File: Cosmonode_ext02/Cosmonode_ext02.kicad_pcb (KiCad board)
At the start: 2 copper layers, 24.1 x 33 mm, 19 parts, among them J1 CONN_01X04, J2 CONN_01X04, J3 CONN_01X08, J4 CONN_01X08, J5 GS3, J6 GS3, Q1 BSS138, Q2 BSS138, SW1 SW_Push, SW2 SW_Push, U1 XC6206P502MR

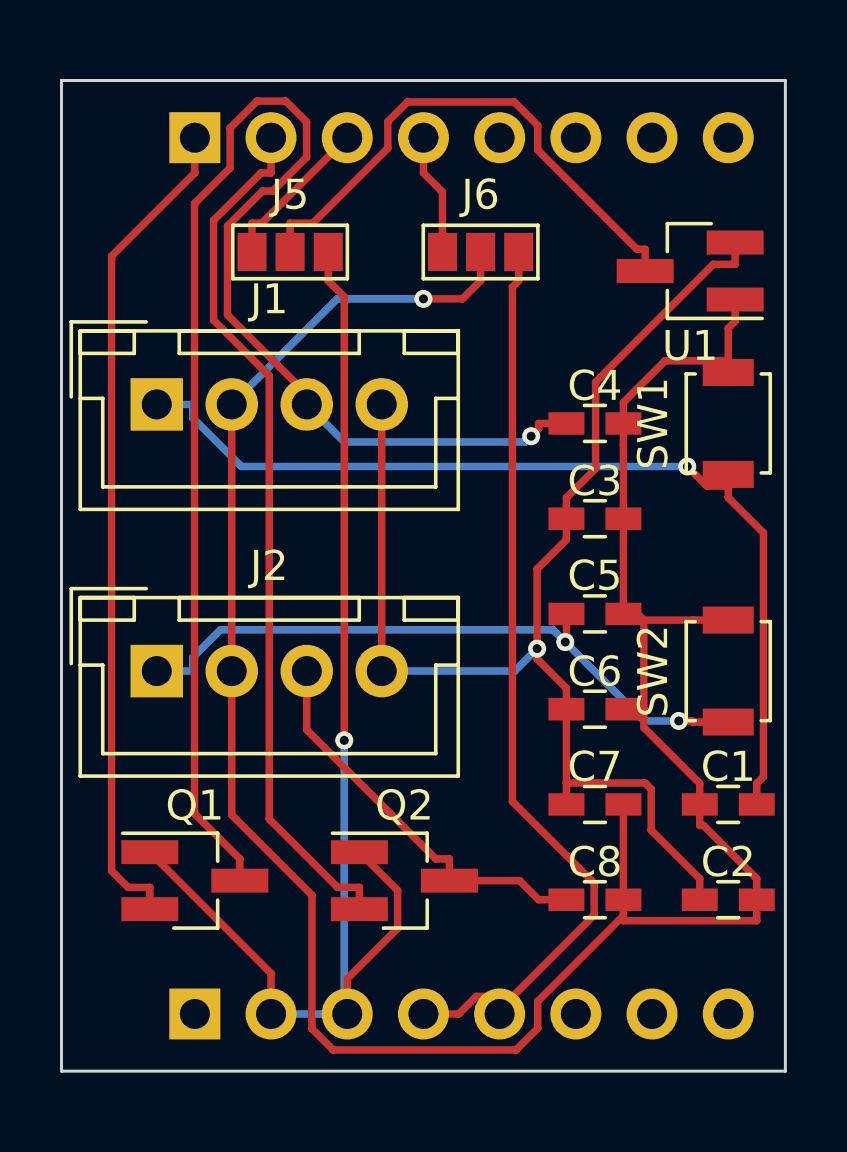
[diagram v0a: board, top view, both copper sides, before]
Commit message: big push!
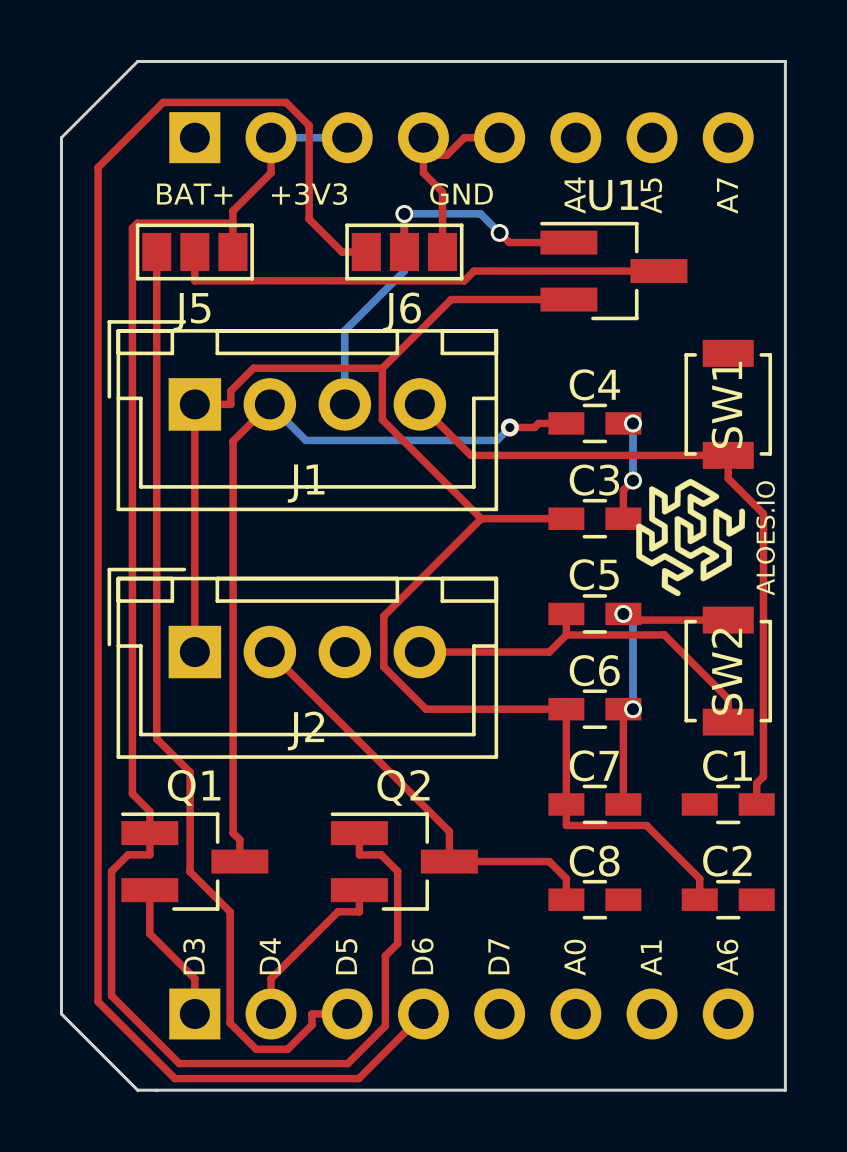
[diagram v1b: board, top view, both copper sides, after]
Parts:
- added J7: Aloes_Logo, Aloes:Aloes_mini, F.Cu at (175.3, 104.8)
- moved J3 29.2 mm to (158.8, 120.7)
- moved J4 29.2 mm to (158.8, 91.4)
- moved J5 3.18 mm to (158.8, 95.2)
- moved J6 2.54 mm to (165.7, 95.2)
- moved U1 2.54 mm to (172.7, 95.9), turned to 0 degrees
- moved J2 1.42 mm to (158.8, 108.6)
- moved J1 1.27 mm to (158.8, 100.3)
- moved Q1 0.64 mm to (158.8, 115.6)
- moved Q2 0.64 mm to (165.7, 115.6)
- moved SW1 0.64 mm to (176.5, 100.3)
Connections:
- net Net-(J3-Pad8) renamed /A6
- net Net-(J4-Pad8) renamed /A7
- J1 pad 1: Net-(C1-Pad2) -> +5V
- J1 pad 2: Net-(C1-Pad1) -> /D3_5V
- J1 pad 3: /D3_5V -> Net-(C1-Pad1)
- J1 pad 4: +5V -> Net-(C1-Pad2)
- J2 pad 1: Net-(C5-Pad2) -> +5V
- J2 pad 2: Net-(C1-Pad1) -> /D4_5V
- J2 pad 3: /D4_5V -> Net-(C1-Pad1)
- J2 pad 4: +5V -> Net-(C5-Pad2)
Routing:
- net Net-(C1-Pad1): track 83.8 -> 28.3 mm, vias 1 -> 6
- net /D6: track 4.07 -> 54.3 mm
- net /D5: track 5.32 -> 31.7 mm
- net /D3_5V: track 50.7 -> 26.5 mm
- net GND: track 31.0 -> 6.86 mm
- net /D4: track 29.1 -> 5.77 mm
- net /D3: track 27.8 -> 4.75 mm
- net +3V3: track 41.8 -> 55.2 mm, vias 1 -> 0
- net +5V: track 43.9 -> 54.4 mm, vias 1 -> 0
- net Net-(C5-Pad2): track 22.1 -> 12.9 mm, vias 2 -> 0
- net Net-(C1-Pad2): track 32.0 -> 23.2 mm, vias 1 -> 0
- net Net-(J5-Pad2): track 18.2 -> 16.6 mm
- net /D4_5V: track 13.4 -> 14.3 mm
- added copper zone on F.Cu, net Net-(C1-Pad1)
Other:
- board size 24.1 x 33 mm -> 24.1 x 34.3 mm
- board text added: "+3V3"
- board text added: "A0"
- board text added: "A1"
- board text added: "A4"
- board text added: "A5"
- board text added: "A6"
- board text added: "A7"
- board text added: "ALOES.IO"
- board text added: "BAT+"
- board text added: "D3"
- board text added: "D4"
- board text added: "D5"
- board text added: "D6"
- board text added: "D7"
- board text added: "GND"
